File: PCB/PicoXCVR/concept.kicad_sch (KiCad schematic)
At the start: 61 parts, among them J1 Antenna, J2 Speaker, J3 Headphone, J4 SSD1306 I2C Display, J5 Conn_01x08_Pin, J6 Conn_01x07_Pin, J7 Conn_01x03, J8 Conn_01x03, SW1 RotaryEncoder_Switch, SW2 SW_Push, SW3 SW_Push, SW4 SW_Push, U1 MCP6022, U2 Pico, U3 74CBTLV3253, U4 74LVC04

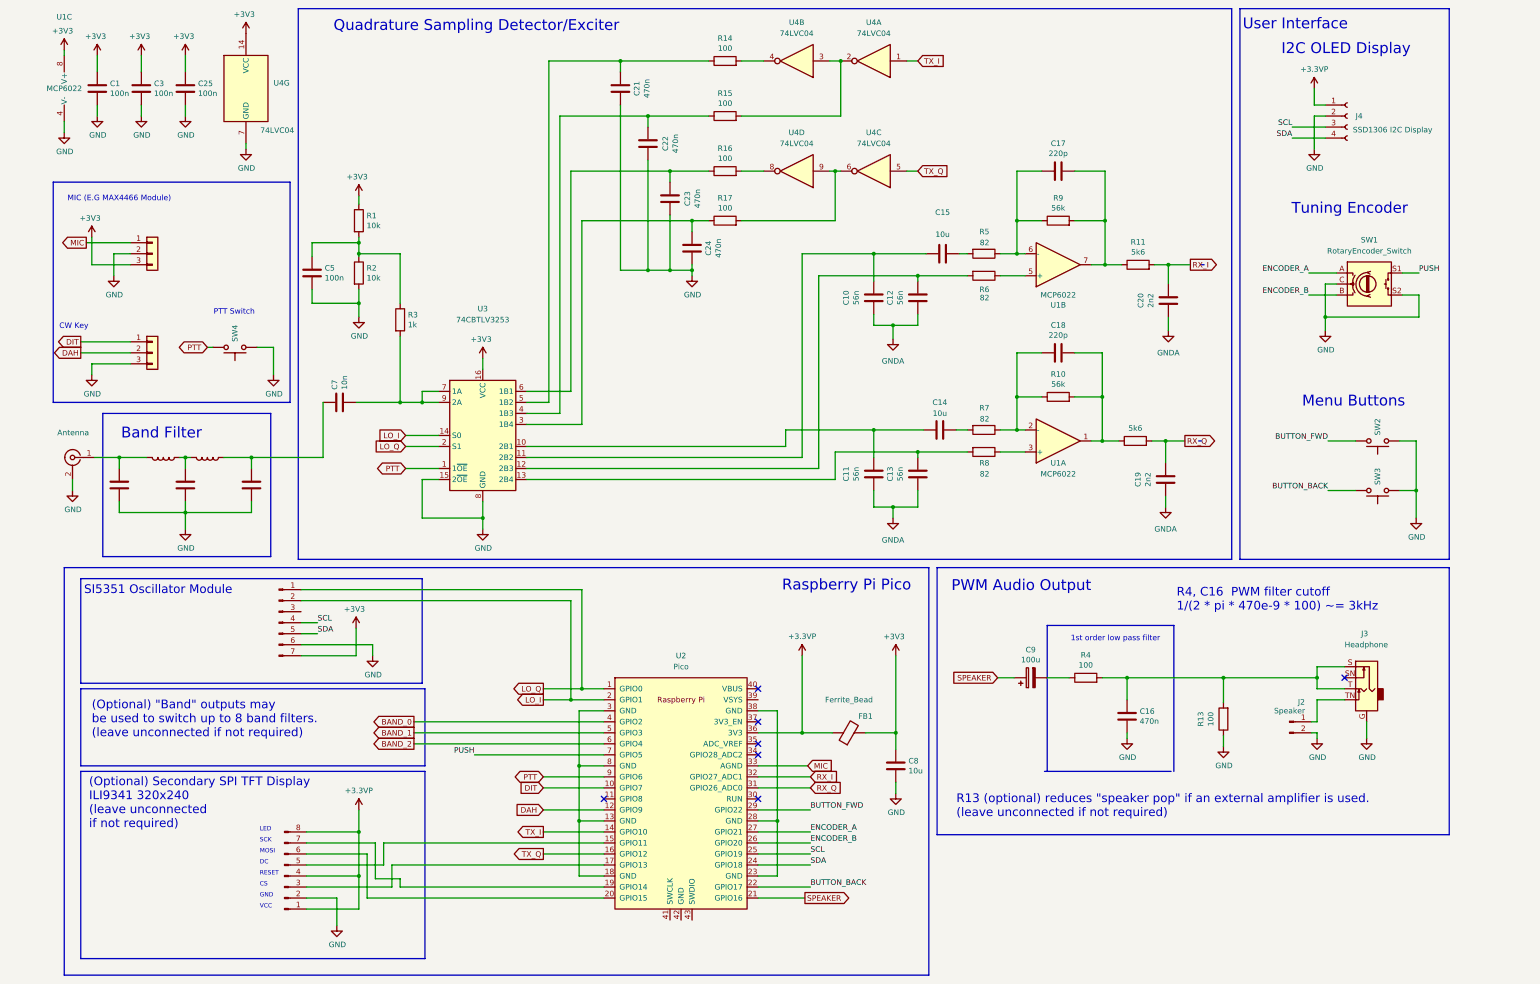
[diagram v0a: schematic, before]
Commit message: latest transceiver experiments
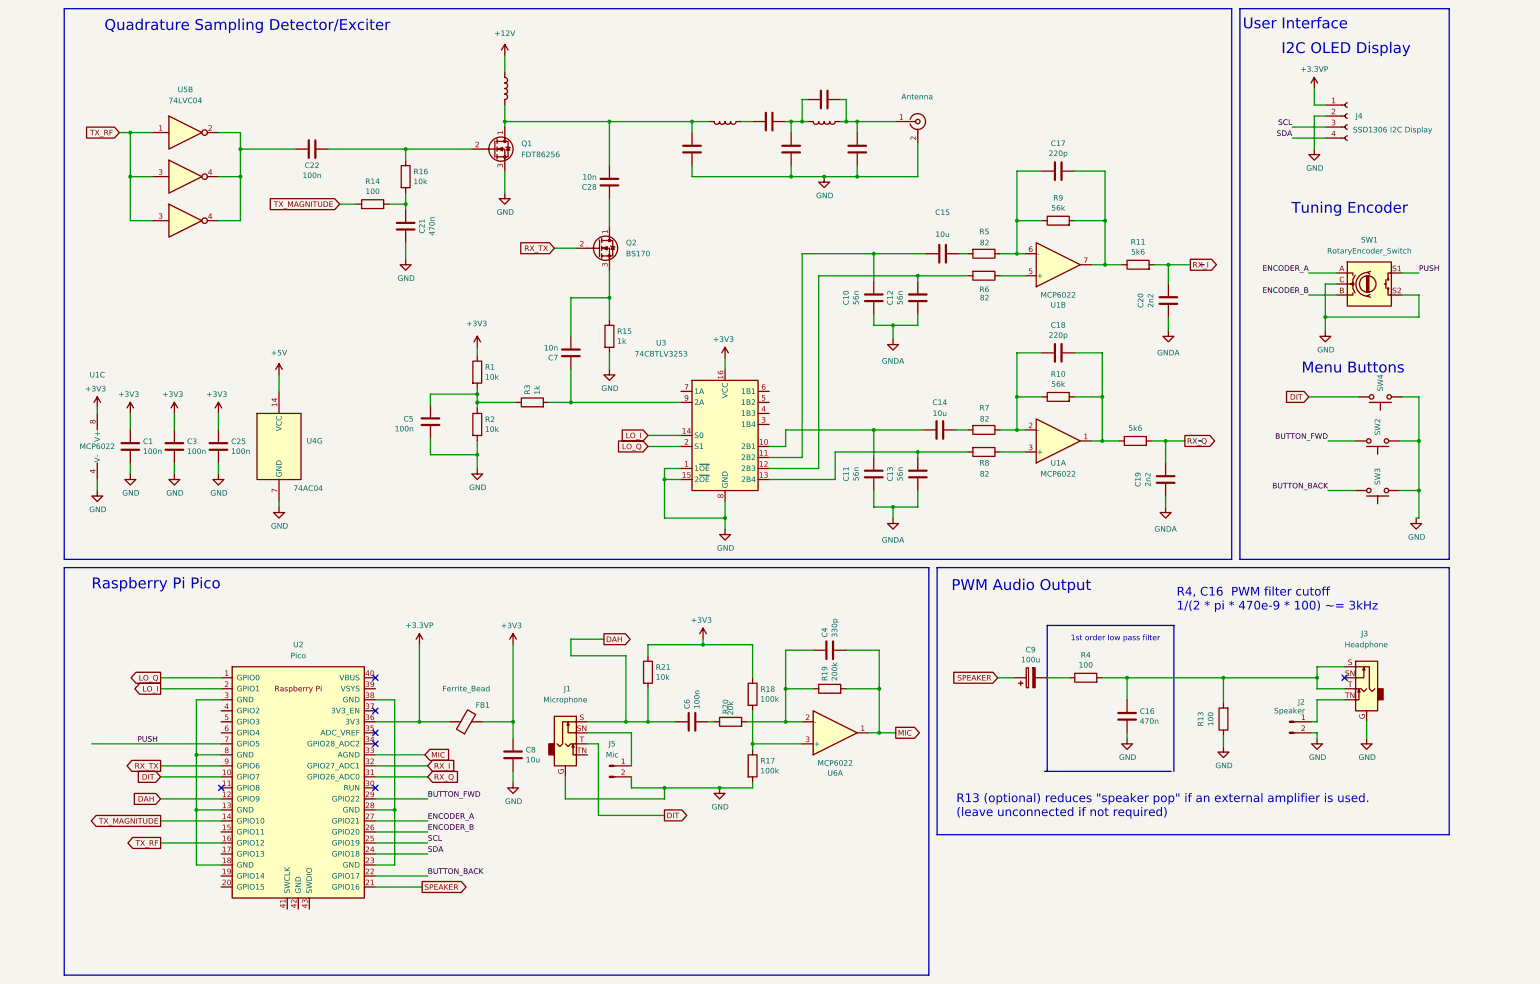
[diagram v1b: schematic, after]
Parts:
- removed J1: Antenna, Connector_Coaxial:SMA_Samtec_SMA-J-P-X-ST-EM1_EdgeMount, symbol Connector:Conn_Coaxial
- removed J5: Conn_01x08_Pin, symbol Connector:Conn_01x08_Pin
- removed J6: Conn_01x07_Pin, symbol Connector:Conn_01x07_Pin
- removed J7, J8: Conn_01x03, symbol Connector_Generic:Conn_01x03
- removed L1, L2: 330n, Inductor_SMD:L_0805_2012Metric_Pad1.05x1.20mm_HandSolder, symbol Device:L
- removed unit 4 of U4
- removed unit 3 of U4
- added C26: 680p, Capacitor_SMD:C_0805_2012Metric, symbol Device:C
- added C27: 1n, Capacitor_SMD:C_0805_2012Metric, symbol Device:C
- added C28: 10n, Capacitor_SMD:C_0805_2012Metric, symbol Device:C
- added J1: Microphone, reciever:jack3.5mm switched, symbol RADIO-rescue:AudioJack2_Ground_Switch-Connector
- added J5: Mic, symbol Connector:Conn_01x02_Pin
- added J9: Antenna, Connector_Coaxial:SMA_Samtec_SMA-J-P-X-ST-EM1_EdgeMount, symbol Connector:Conn_Coaxial
- added L3, L4, L5: 330n, Inductor_SMD:L_0805_2012Metric_Pad1.05x1.20mm_HandSolder, symbol Device:L
- added Q1: FDT86256, Package_TO_SOT_THT:TO-92_Inline, symbol Transistor_FET:BS170
- added Q2: BS170, Package_TO_SOT_THT:TO-92_Inline, symbol Transistor_FET:BS170
- added R18: 100k, Resistor_SMD:R_0805_2012Metric, symbol Device:R
- added R19: 200k, Resistor_SMD:R_0805_2012Metric, symbol Device:R
- added R20: 20k, Resistor_SMD:R_0805_2012Metric, symbol Device:R
- added R21: 10k, Resistor_SMD:R_0805_2012Metric, symbol Device:R
- added U5: 74LVC04, symbol 74xx:74LS04
- added U6: MCP6022, Package_SO:MSOP-8-1EP_3x3mm_P0.65mm_EP1.68x1.88mm, symbol Amplifier_Operational:LM4562
- C22: value 470n -> 100n
- C23: value 470n -> 1n
- C24: value 470n -> 680p
- C4: value 1n -> 330p
- C6: value 680p -> 100n
- R15: value 100 -> 1k
- R16: value 100 -> 10k
- R17: value 100 -> 100k
- U4: value 74LVC04 -> 74AC04
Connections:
- net +3V3: now also R18.1, R21.1; no longer U4.14 (VCC)
- net DAH: now also C6.1, J1.S, R21.2
- net DIT: now also SW4.2, J1.T
- net GND: now also R15.2, R17.2, U3.1 (1~{OE}), C26.1, J1.G, J5.2 (Pin_2), J9.2 (Ext), Q1.3 (S); no longer C22.1, C23.1, C4.1, C6.1
- net MIC: now also C4.2, R19.2, U6.1
- net at U4.4: now also C22.1, U4.2, U5.4; no longer R14.2
- net at R16.2: now also C21.2, R14.2
- net at C6.2: now also R20.1; no longer C7.1
- net at R3.2, U3.9 (2A): now also C7.1; no longer C7.2, U3.7 (1A)
- net at C2.2: now also C28.2, L3.2, L4.2, Q1.1 (D)
- net BAND_0: no longer names the net of U2.4 (GPIO2)
- net BAND_1: no longer names the net of U2.5 (GPIO3)
- net BAND_2: no longer names the net of U2.6 (GPIO4)
- removed net PTT: SW4.2, U2.9 (GPIO6), U3.1 (1~{OE})
- net TX_I renamed TX_MAGNITUDE
- net TX_MAGNITUDE: now also R14.1; no longer U4.1
- net TX_Q renamed TX_RF
- net TX_RF: now also U4.1, U4.3, U5.3
- new net: R17.1, R18.2, U6.3 (+)
- new net: C4.1, R19.1, R20.2, U6.2 (-)
- new net: C23.2, L4.1
- new net: J1.SN, J5.1 (Pin_1)
- new net: C24.2, C27.1, J9.1 (In), L5.1
- new net: C7.2, Q2.3 (S), R15.1
- new net: C28.1, Q2.1 (D)
- new net: C22.2, Q1.2 (G), R16.1
- new net: C23.1, C26.2, C27.2, L5.2
- new net +12V: L3.1
- new net +5V: U4.14 (VCC)
- new net RX_TX: Q2.2 (G), U2.9 (GPIO6)
- now unconnected: U3.3 (1B4), U3.4 (1B3), U3.5 (1B2), U3.6 (1B1)
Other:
- note removed: "(Optional) "Band" outputs may be used to switch up to 8 band filters. (leave unconnected if not required)"
- note removed: "(Optional) Secondary SPI TFT Display ILI9341 320x240 (leave unconnected if not required)"
- note removed: "Band Filter"
- note removed: "CS"
- note removed: "CW Key"
- note removed: "DC"
- note removed: "GND"
- note removed: "LED"
- note removed: "MIC (E.G MAX4466 Module)"
- note removed: "MOSI"
- note removed: "PTT Switch"
- note removed: "RESET"
- note removed: "SCK"
- note removed: "SI5351 Oscillator Module"
- note removed: "VCC"
- moved on the sheet: C1, C21, C25, C3, C5, C7, C8, FB1, R1, R14, R2, R3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
